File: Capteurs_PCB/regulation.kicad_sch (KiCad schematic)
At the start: 23 parts, among them U2 AZ1117-3.3

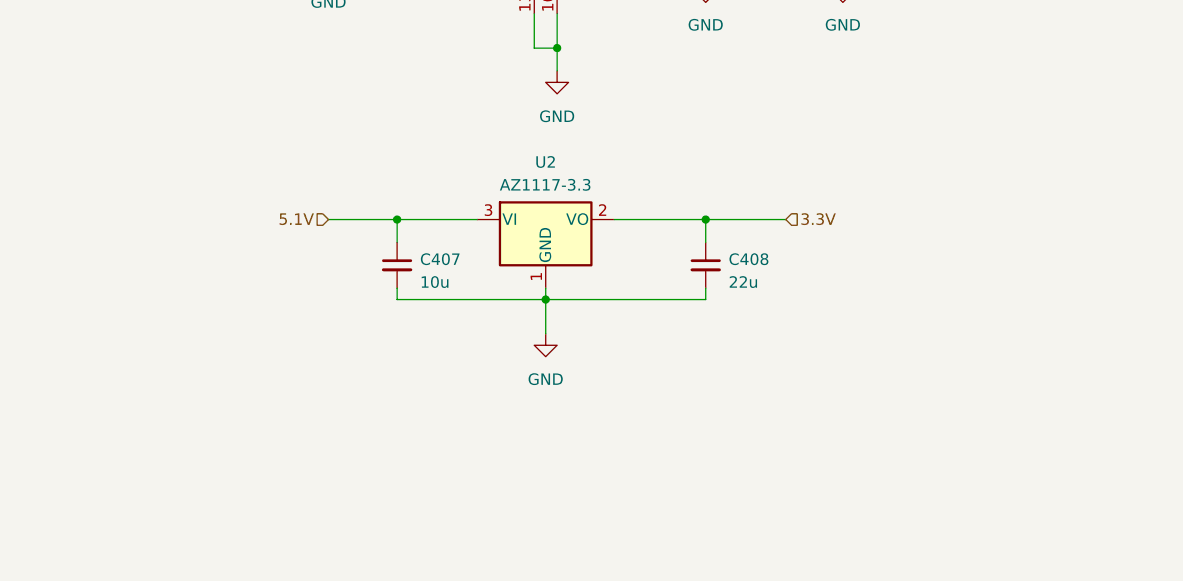
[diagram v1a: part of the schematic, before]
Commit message: Footprint design and Footprint assignment
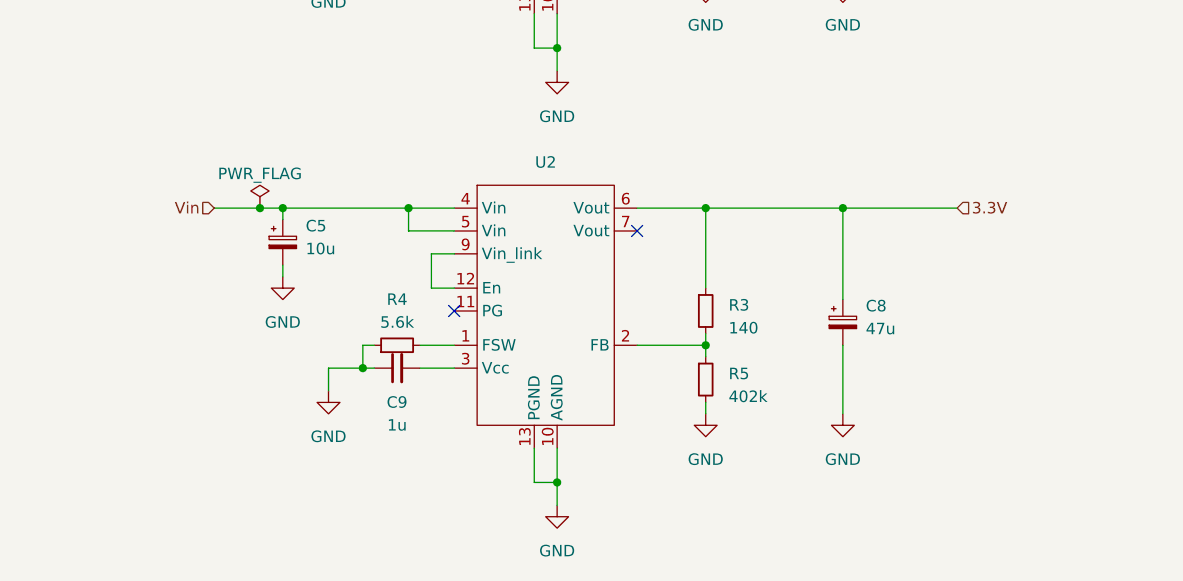
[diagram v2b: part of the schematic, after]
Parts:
- removed C407: 10u, Capacitor_SMD:C_1206_3216Metric_Pad1.33x1.80mm_HandSolder, symbol Device:C_Small
- removed C408: 22u, Capacitor_SMD:C_1206_3216Metric_Pad1.33x1.80mm_HandSolder, symbol Device:C_Small
- removed U2: AZ1117-3.3, Package_TO_SOT_THT:TO-220-3_Vertical, symbol Regulator_Linear:AZ1117-3.3
- added C5: 10u, Capacitor_SMD:CP_Elec_5x5.4, symbol Device:C_Polarized_Small
- added C8: 47u, Capacitor_SMD:CP_Elec_6.3x5.4, symbol Device:C_Polarized_Small
- added C9: 1u, Capacitor_SMD:C_1206_3216Metric_Pad1.33x1.80mm_HandSolder, symbol Device:C_Small
- added R3: 140, Resistor_SMD:R_0603_1608Metric_Pad0.98x0.95mm_HandSolder, symbol Device:R_Small
- added R4: 5.6k, Resistor_SMD:R_0603_1608Metric_Pad0.98x0.95mm_HandSolder, symbol Device:R_Small
- added R5: 402k, Resistor_SMD:R_0603_1608Metric_Pad0.98x0.95mm_HandSolder, symbol Device:R_Small
- added U2: ~, Custom:Regulator, symbol custom:171013801
- U401, U402: footprint (none) -> Custom:Regulator
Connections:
- net 3.3V: now also C8.1, R3.1, U2.6 (Vout)
- net GND: now also C5.2, C8.2, C9.1, R4.1, R5.2, U2.10 (AGND), U2.13 (PGND)
- net Vin: now also C5.1, U2.4 (Vin), U2.5 (Vin)
- new net: C9.2, U2.3 (Vcc)
- new net: R4.2, U2.1 (FSW)
- new net: U2.12 (En), U2.9 (Vin_link)
- new net: R3.2, R5.1, U2.2 (FB)
- no-connect marks 4 -> 6
